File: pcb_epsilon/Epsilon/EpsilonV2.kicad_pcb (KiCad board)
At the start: 2 copper layers, 29 x 11.5 mm, 18 parts, among them J1 SG1m, J2 SG2p, J3 SG1p, J4 SG2m, Q1 AO3401A, U1 ADA4940-1ARZ-R7, U2 DS28E07P+T

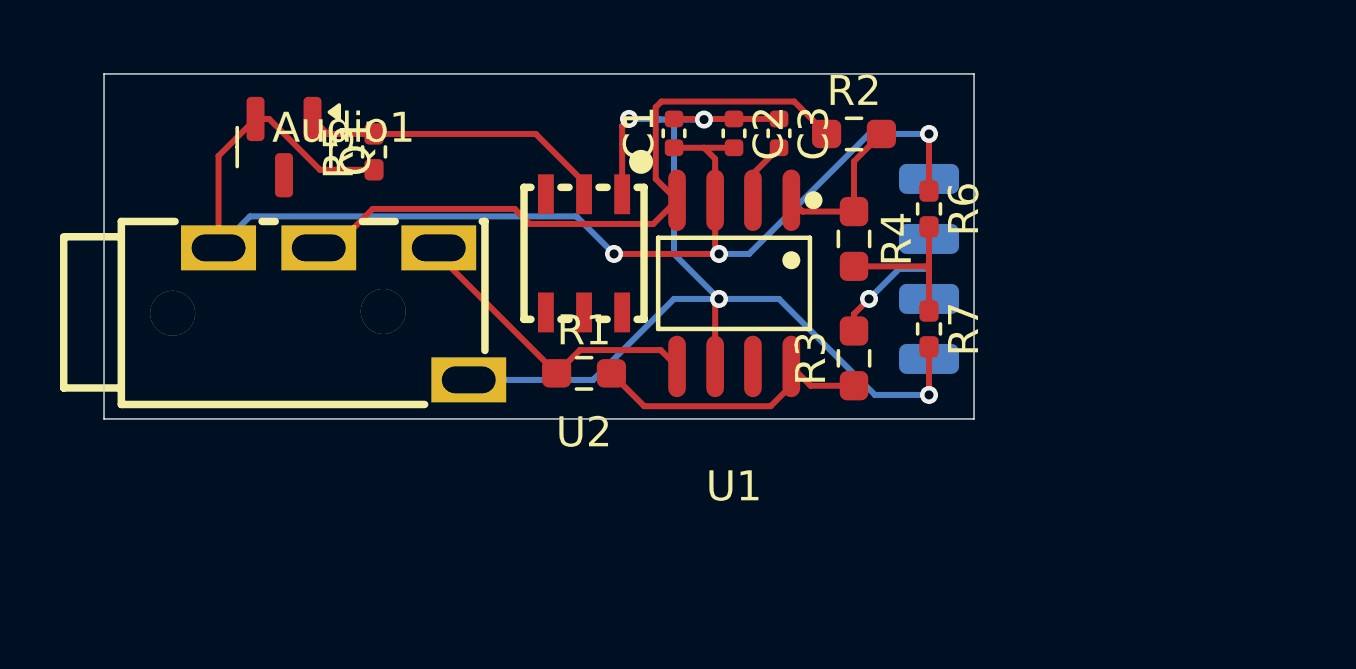
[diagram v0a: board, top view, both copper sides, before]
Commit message: Yolo
Nothing could go wrong
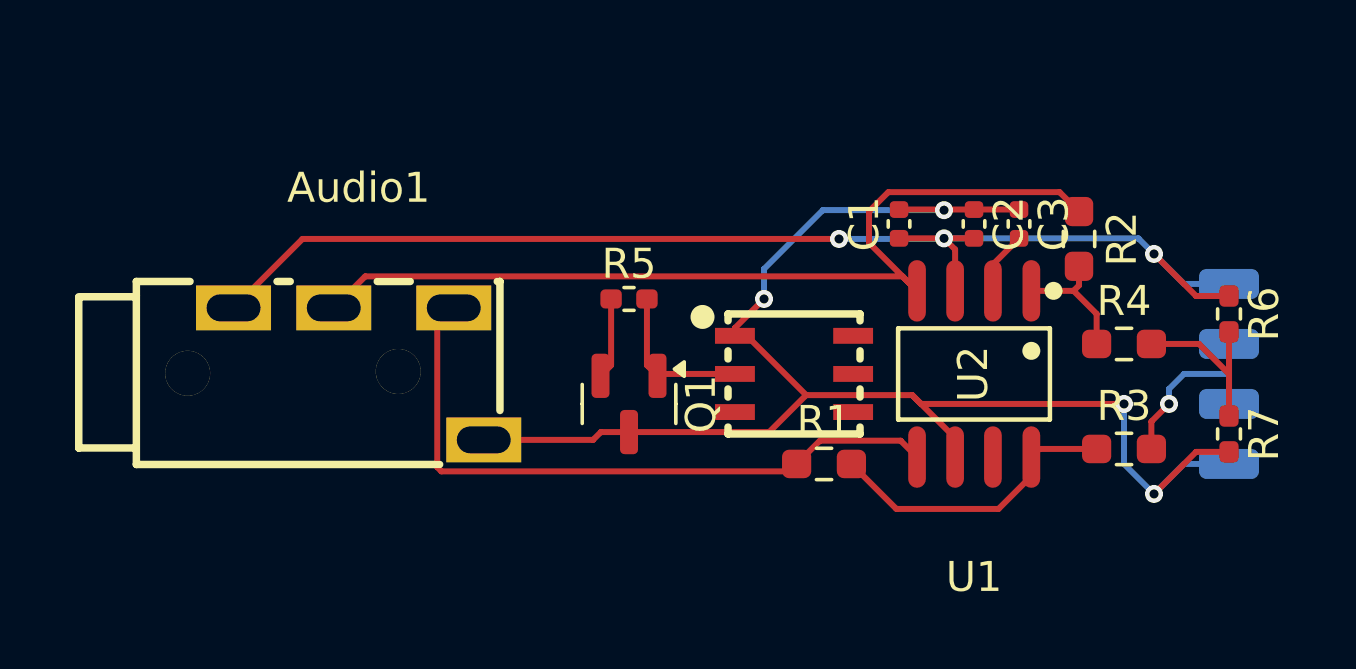
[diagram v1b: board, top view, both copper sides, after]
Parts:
- moved Q1 14.3 mm to (159.0, 131.0)
- moved J1 10.6 mm to (179.0, 129.0)
- moved J2 10.6 mm to (179.0, 131.0)
- moved J3 10.6 mm to (179.0, 127.0)
- moved J4 10.6 mm to (179.0, 133.0)
- moved R6 10.6 mm to (179.0, 128.0)
- moved R7 10.6 mm to (179.0, 132.0)
- moved R5 9.81 mm to (159.0, 127.5), turned to 0 degrees
- moved R4 9.66 mm to (175.5, 129.0), turned to 0 degrees
- moved R3 9.49 mm to (175.5, 132.5), turned to 0 degrees
- moved R1 8.55 mm to (165.5, 133.0)
- moved C2 8.55 mm to (170.5, 125.0)
- moved C3 8.55 mm to (172.0, 125.0)
- moved U1 8.55 mm to (170.5, 130.0)
- moved R2 8.28 mm to (174.0, 125.5), turned to -90 degrees
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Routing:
- net GND: track 38.1 -> 50.8 mm
- net Net-(U1-–OUT): track 10.4 -> 22.2 mm
- net Net-(U1-+OUT): track 22.6 -> 30.9 mm
- net Net-(Q1-G): track 10.3 -> 5.31 mm
- net Net-(U1-–IN): track 5.21 -> 4.39 mm
- net Net-(J1-Pin_1): track 5.69 -> 6.45 mm
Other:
- board outline removed
